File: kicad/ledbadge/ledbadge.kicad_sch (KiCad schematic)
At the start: 10 parts, among them J1 AVR-ISP-6, J2 Conn_01x02, SW1 SW_SPST, U1 ATtiny85-20P

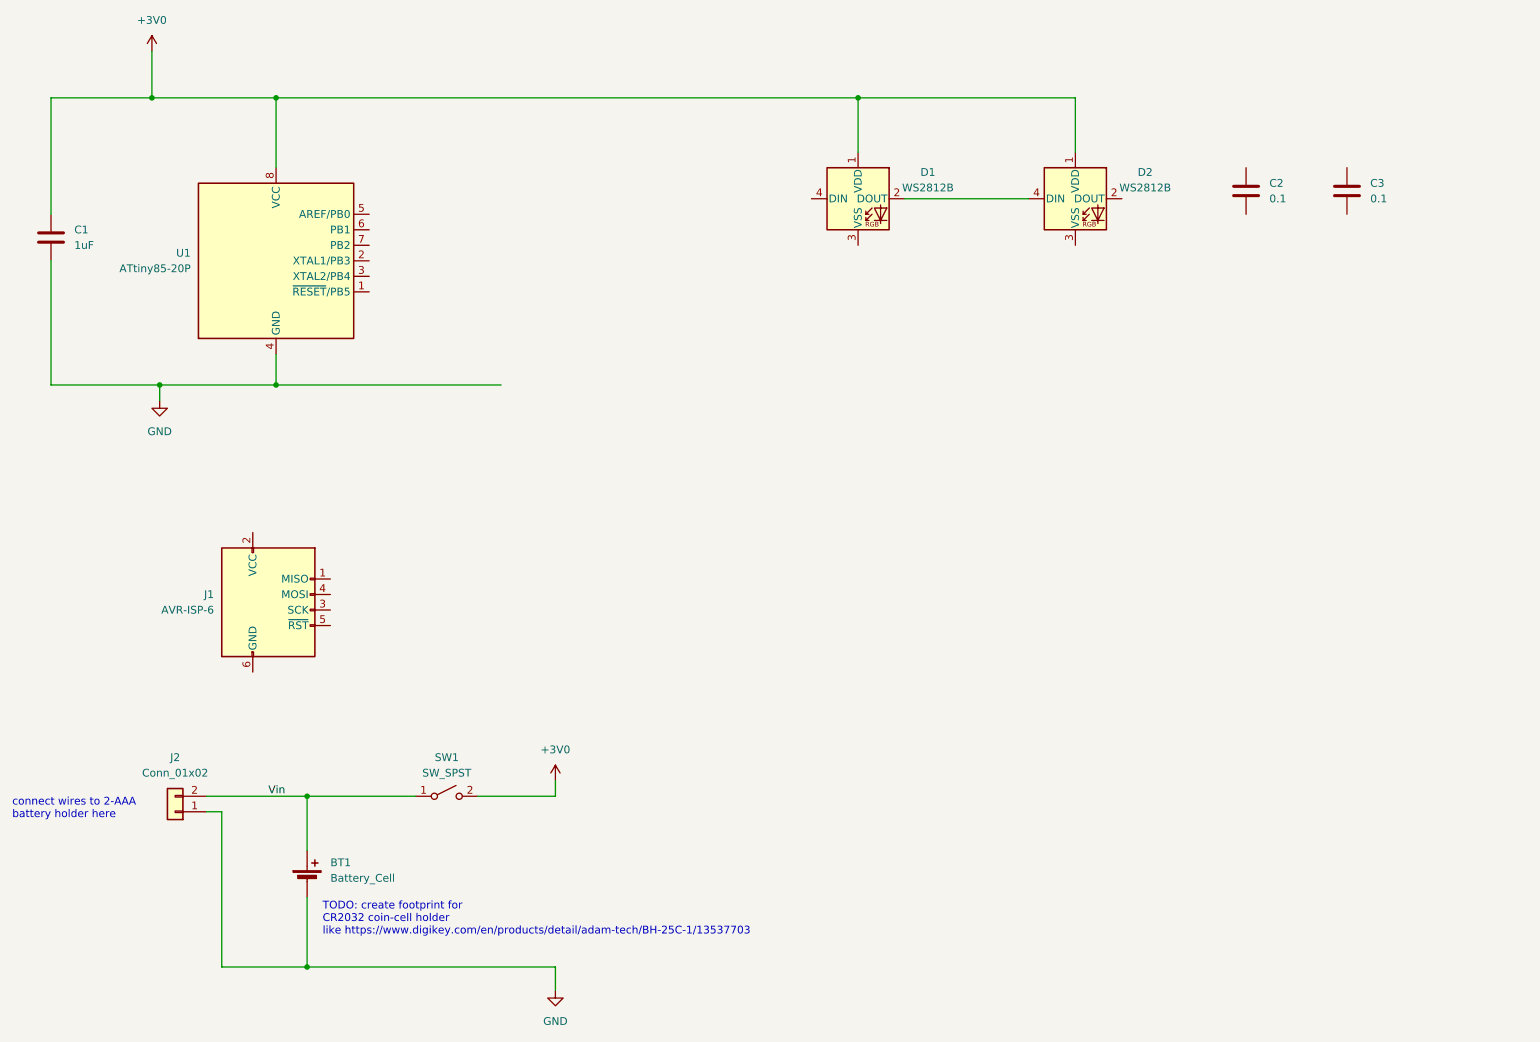
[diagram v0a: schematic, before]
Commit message: add symbols, commit some of my text notes rest of the symbols that we definitely need decide to add rough notes for easier sync with laptop, ahead of cleaning up into nice md files
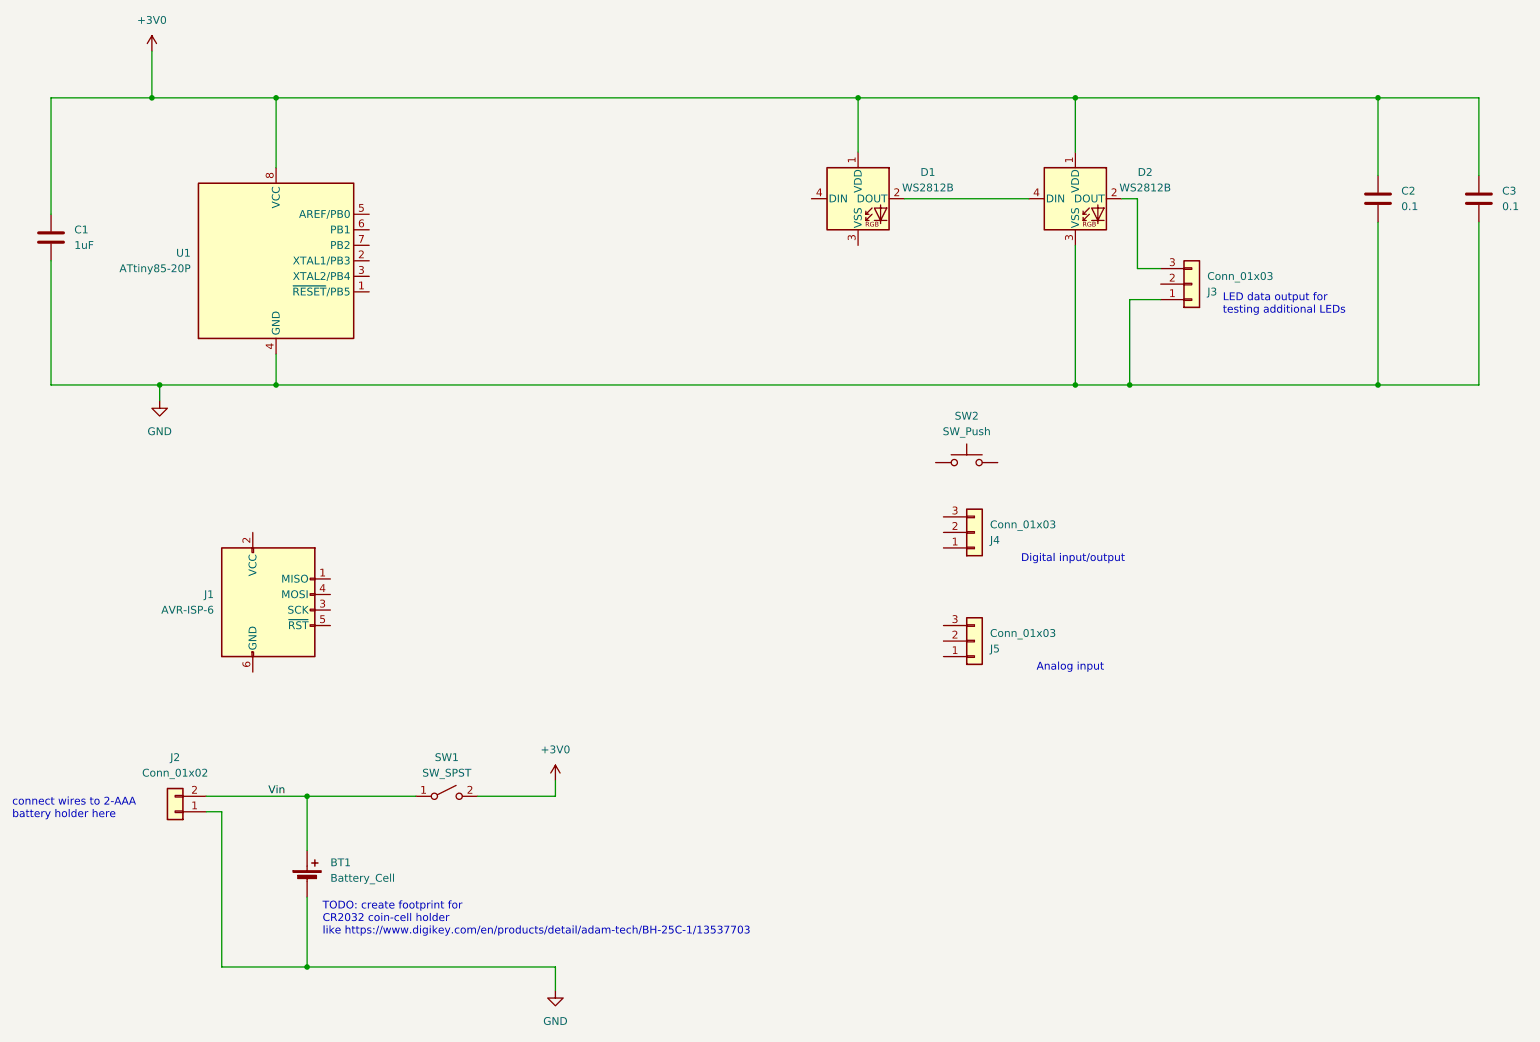
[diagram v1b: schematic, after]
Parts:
- added J3, J4, J5: Conn_01x03, symbol Connector_Generic:Conn_01x03
- added SW2: SW_Push, symbol Switch:SW_Push
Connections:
- net +3V0: now also C2.1, C3.1
- net GND: now also C2.2, C3.2, D2.3 (VSS), J3.1 (Pin_1)
- net at D2.2 (DOUT): now also J3.3 (Pin_3)
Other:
- note added: "Analog input"
- note added: "Digital input/output"
- note added: "LED data output for testing additional LEDs"
- moved on the sheet: C2, C3
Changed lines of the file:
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@@
   (junction (at 68.58 40.64) (diameter 0) (color 0 0 0 0)
   )
+  (junction (at 199.39 40.64) (diameter 0) (color 0 0 0 0)
+  )
   (junction (at 163.83 40.64) (diameter 0) (color 0 0 0 0)
   )
   (junction (at 68.58 87.63) (diameter 0) (color 0 0 0 0)
   )
+  (junction (at 248.92 40.64) (diameter 0) (color 0 0 0 0)
+  )
+  (junction (at 199.39 87.63) (diameter 0) (color 0 0 0 0)
+  )
   (junction (at 48.26 40.64) (diameter 0) (color 0 0 0 0)
   )
+  (junction (at 208.28 87.63) (diameter 0) (color 0 0 0 0)
+  )
+  (junction (at 248.92 87.63) (diameter 0) (color 0 0 0 0)
+  )
   (wire (pts (xy 73.66 154.94) (xy 91.44 154.94))
     (stroke (width 0) (type default))
@@
     (stroke (width 0) (type default))
   )
-  (wire (pts (xy 68.58 87.63) (xy 105.41 87.63))
+  (wire (pts (xy 68.58 87.63) (xy 199.39 87.63))
+    (stroke (width 0) (type default))
+  )
+  (wire (pts (xy 248.92 87.63) (xy 265.43 87.63))
     (stroke (width 0) (type default))
   )
@@
     (stroke (width 0) (type default))
   )
+  (wire (pts (xy 199.39 87.63) (xy 208.28 87.63))
+    (stroke (width 0) (type default))
+  )
   (wire (pts (xy 59.69 157.48) (xy 59.69 182.88))
     (stroke (width 0) (type default))
@@
     (stroke (width 0) (type default))
   )
+  (wire (pts (xy 208.28 87.63) (xy 248.92 87.63))
+    (stroke (width 0) (type default))
+  )
   (wire (pts (xy 68.58 40.64) (xy 163.83 40.64))
     (stroke (width 0) (type default))
@@
     (stroke (width 0) (type default))
   )
+  (wire (pts (xy 248.92 40.64) (xy 265.43 40.64))
+    (stroke (width 0) (type default))
+  )
   (wire (pts (xy 114.3 152.4) (xy 114.3 154.94))
     (stroke (width 0) (type default))
   )
+  (wire (pts (xy 265.43 87.63) (xy 265.43 60.96))
+    (stroke (width 0) (type default))
+  )
+  (wire (pts (xy 208.28 87.63) (xy 208.28 73.66))
+    (stroke (width 0) (type default))
+  )
   (wire (pts (xy 73.66 154.94) (xy 73.66 163.83))
     (stroke (width 0) (type default))
@@
     (stroke (width 0) (type default))
   )
+  (wire (pts (xy 207.01 57.15) (xy 209.55 57.15))
+    (stroke (width 0) (type default))
+  )
   (wire (pts (xy 57.15 157.48) (xy 59.69 157.48))
     (stroke (width 0) (type default))
   )
+  (wire (pts (xy 248.92 40.64) (xy 248.92 53.34))
+    (stroke (width 0) (type default))
+  )
+  (wire (pts (xy 209.55 57.15) (xy 209.55 68.58))
+    (stroke (width 0) (type default))
+  )
   (wire (pts (xy 199.39 49.53) (xy 199.39 40.64))
     (stroke (width 0) (type default))
@@
     (stroke (width 0) (type default))
   )
+  (wire (pts (xy 199.39 87.63) (xy 199.39 64.77))
+    (stroke (width 0) (type default))
+  )
   (wire (pts (xy 163.83 40.64) (xy 199.39 40.64))
     (stroke (width 0) (type default))
@@
     (stroke (width 0) (type default))
   )
+  (wire (pts (xy 199.39 40.64) (xy 248.92 40.64))
+    (stroke (width 0) (type default))
+  )
   (wire (pts (xy 171.45 57.15) (xy 191.77 57.15))
     (stroke (width 0) (type default))
   )
+  (wire (pts (xy 208.28 73.66) (xy 213.36 73.66))
+    (stroke (width 0) (type default))
+  )
+  (wire (pts (xy 209.55 68.58) (xy 213.36 68.58))
+    (stroke (width 0) (type default))
+  )
   (wire (pts (xy 59.69 182.88) (xy 73.66 182.88))
     (stroke (width 0) (type default))
@@
   (wire (pts (xy 163.83 40.64) (xy 163.83 49.53))
     (stroke (width 0) (type default))
+  )
+  (wire (pts (xy 265.43 40.64) (xy 265.43 53.34))
+    (stroke (width 0) (type default))
+  )
+  (wire (pts (xy 248.92 87.63) (xy 248.92 60.96))
+    (stroke (width 0) (type default))
+  )
+  (text "Analog input" (at 193.04 134.62 0)
+    (effects (font (size 1.27 1.27)) (justify left bottom))
   )
   (text "TODO: create footprint for\nCR2032 coin-cell holder\nlike https://www.digikey.com/en/products/detail/adam-tech/BH-25C-1/13537703"
@@
   )
   (text "connect wires to 2-AAA\nbattery holder here" (at 25.4 158.75 0)
+    (effects (font (size 1.27 1.27)) (justify left bottom))
+  )
+  (text "Digital input/output" (at 190.5 116.84 0)
+    (effects (font (size 1.27 1.27)) (justify left bottom))
+  )
+  (text "LED data output for \ntesting additional LEDs" (at 223.52 76.2 0)
     (effects (font (size 1.27 1.27)) (justify left bottom))
   )
@@
         (path "/3a89a026-2e2f-4a4d-a795-8a4846df971d"
           (reference "SW1") (unit 1)
+        )
+      )
+    )
+  )
+  (symbol (lib_id "Connector_Generic:Conn_01x03") (at 182.88 129.54 0) (mirror x) (unit 1)
+    (in_bom yes) (on_board yes) (dnp no)
+    (property "Reference" "J5" (at 185.42 130.81 0)
+      (effects (font (size 1.27 1.27)) (justify left))
+    )
+    (property "Value" "Conn_01x03" (at 185.42 128.27 0)
+      (effects (font (size 1.27 1.27)) (justify left))
+    )
+    (property "Footprint" "" (at 182.88 129.54 0)
+      (effects (font (size 1.27 1.27)) hide)
+    )
+    (property "Datasheet" "~" (at 182.88 129.54 0)
+      (effects (font (size 1.27 1.27)) hide)
+    )
+    (pin "3")
+    (pin "2")
+    (pin "1")
+    (instances
+      (project "ledbadge"
+        (path "/3a89a026-2e2f-4a4d-a795-8a4846df971d"
+          (reference "J5") (unit 1)
         )
       )
@@
     )
   )
+  (symbol (lib_id "Switch:SW_Push") (at 181.61 100.33 0) (unit 1)
+    (in_bom yes) (on_board yes) (dnp no)
+    (property "Reference" "SW2" (at 181.61 92.71 0)
+      (effects (font (size 1.27 1.27)))
+    )
+    (property "Value" "SW_Push" (at 181.61 95.25 0)
+      (effects (font (size 1.27 1.27)))
+    )
+    (property "Footprint" "" (at 181.61 95.25 0)
+      (effects (font (size 1.27 1.27)) hide)
+    )
+    (property "Datasheet" "~" (at 181.61 95.25 0)
+      (effects (font (size 1.27 1.27)) hide)
+    )
+    (pin "2")
+    (pin "1")
+    (instances
+      (project "ledbadge"
+        (path "/3a89a026-2e2f-4a4d-a795-8a4846df971d"
+          (reference "SW2") (unit 1)
+        )
+      )
+    )
+  )
   (symbol (lib_id "power:GND") (at 114.3 186.69 0) (unit 1)
     (in_bom yes) (on_board yes) (dnp no) (fields_autoplaced)
@@
     )
   )
-  (symbol (lib_id "Device:C") (at 227.33 55.88 0) (unit 1)
-    (in_bom yes) (on_board yes) (dnp no) (fields_autoplaced)
-    (property "Reference" "C2" (at 231.14 54.61 0)
-      (effects (font (size 1.27 1.27)) (justify left))
-    )
-    (property "Value" "0.1" (at 231.14 57.15 0)
-      (effects (font (size 1.27 1.27)) (justify left))
-    )
-    (property "Footprint" "" (at 228.2952 59.69 0)
-      (effects (font (size 1.27 1.27)) hide)
-    )
-    (property "Datasheet" "~" (at 227.33 55.88 0)
+  (symbol (lib_id "Connector_Generic:Conn_01x03") (at 182.88 111.76 0) (mirror x) (unit 1)
+    (in_bom yes) (on_board yes) (dnp no)
+    (property "Reference" "J4" (at 185.42 113.03 0)
+      (effects (font (size 1.27 1.27)) (justify left))
+    )
+    (property "Value" "Conn_01x03" (at 185.42 110.49 0)
+      (effects (font (size 1.27 1.27)) (justify left))
+    )
+    (property "Footprint" "" (at 182.88 111.76 0)
+      (effects (font (size 1.27 1.27)) hide)
+    )
+    (property "Datasheet" "~" (at 182.88 111.76 0)
+      (effects (font (size 1.27 1.27)) hide)
+    )
+    (pin "1")
+    (pin "3")
+    (pin "2")
+    (instances
+      (project "ledbadge"
+        (path "/3a89a026-2e2f-4a4d-a795-8a4846df971d"
+          (reference "J4") (unit 1)
+        )
+      )
+    )
+  )
+  (symbol (lib_id "Device:C") (at 248.92 57.15 0) (unit 1)
+    (in_bom yes) (on_board yes) (dnp no) (fields_autoplaced)
+    (property "Reference" "C2" (at 252.73 55.88 0)
+      (effects (font (size 1.27 1.27)) (justify left))
+    )
+    (property "Value" "0.1" (at 252.73 58.42 0)
+      (effects (font (size 1.27 1.27)) (justify left))
+    )
+    (property "Footprint" "" (at 249.8852 60.96 0)
+      (effects (font (size 1.27 1.27)) hide)
+    )
+    (property "Datasheet" "~" (at 248.92 57.15 0)
       (effects (font (size 1.27 1.27)) hide)
     )
@@
     )
   )
-  (symbol (lib_id "Device:C") (at 243.84 55.88 0) (unit 1)
-    (in_bom yes) (on_board yes) (dnp no) (fields_autoplaced)
-    (property "Reference" "C3" (at 247.65 54.61 0)
-      (effects (font (size 1.27 1.27)) (justify left))
-    )
-    (property "Value" "0.1" (at 247.65 57.15 0)
-      (effects (font (size 1.27 1.27)) (justify left))
-    )
-    (property "Footprint" "" (at 244.8052 59.69 0)
-      (effects (font (size 1.27 1.27)) hide)
-    )
-    (property "Datasheet" "~" (at 243.84 55.88 0)
+  (symbol (lib_id "Device:C") (at 265.43 57.15 0) (unit 1)
+    (in_bom yes) (on_board yes) (dnp no) (fields_autoplaced)
+    (property "Reference" "C3" (at 269.24 55.88 0)
+      (effects (font (size 1.27 1.27)) (justify left))
+    )
+    (property "Value" "0.1" (at 269.24 58.42 0)
+      (effects (font (size 1.27 1.27)) (justify left))
+    )
+    (property "Footprint" "" (at 266.3952 60.96 0)
+      (effects (font (size 1.27 1.27)) hide)
+    )
+    (property "Datasheet" "~" (at 265.43 57.15 0)
       (effects (font (size 1.27 1.27)) hide)
     )
@@
         )
       )
+    )
+  )
+  (symbol (lib_id "Connector_Generic:Conn_01x03") (at 218.44 71.12 0) (mirror x) (unit 1)
+    (in_bom yes) (on_board yes) (dnp no)
+    (property "Reference" "J3" (at 220.98 72.39 0)
+      (effects (font (size 1.27 1.27)) (justify left))
+    )
+    (property "Value" "Conn_01x03" (at 220.98 69.85 0)
+      (effects (font (size 1.27 1.27)) (justify left))
+    )
+    (property "Footprint" "" (at 218.44 71.12 0)
+      (effects (font (size 1.27 1.27)) hide)
+    )
+    (property "Datasheet" "~" (at 218.44 71.12 0)
+      (effects (font (size 1.27 1.27)) hide)
+    )
+    (pin "2")
+    (pin "1")
+    (pin "3")
+    (instances
+      (project "ledbadge"
+        (path "/3a89a026-2e2f-4a4d-a795-8a4846df971d"
+          (reference "J3") (unit 1)
+        )
+      )
